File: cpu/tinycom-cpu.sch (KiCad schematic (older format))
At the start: 10 parts, among them P1 CONN_02X08, P2 CONN_02X08, U1 OLIMEX_IC_A13, U2 H5TQ2G83BFR/FBGA82, Y1 Crystal

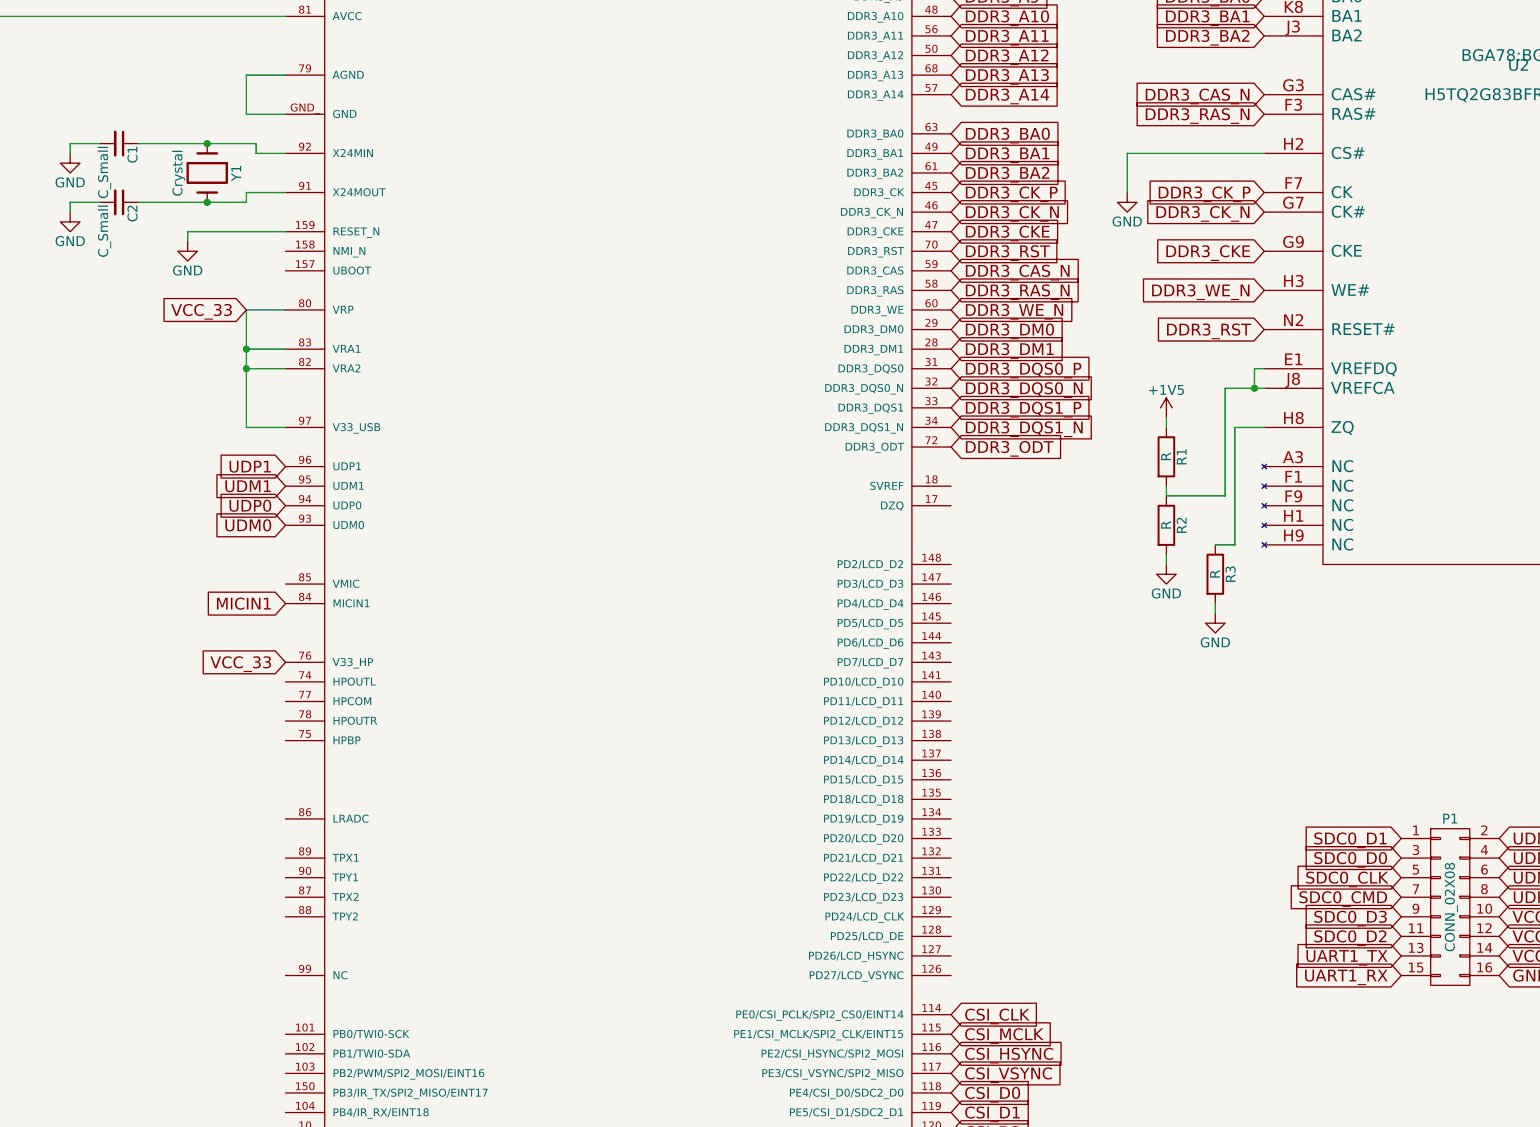
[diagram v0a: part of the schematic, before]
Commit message: router power
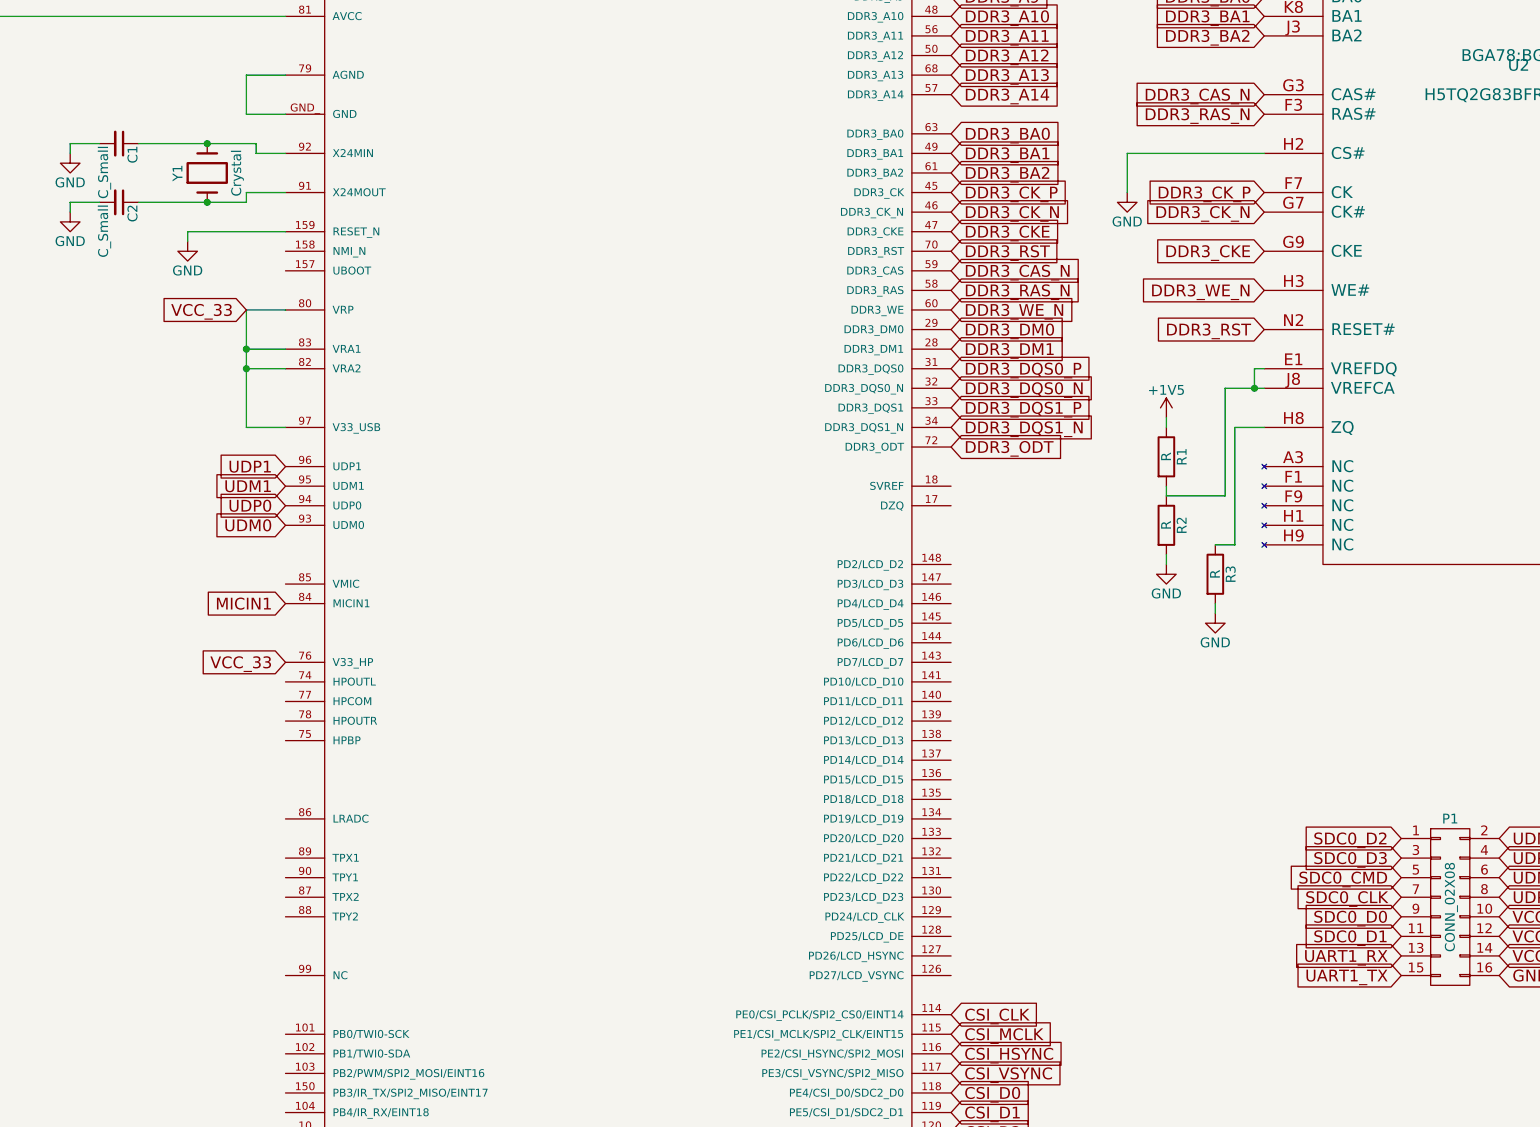
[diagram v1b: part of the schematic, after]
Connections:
- net SDC0_CLK: now also P1.7 (P7); no longer P1.5 (P5)
- net SDC0_CMD: now also P1.5 (P5); no longer P1.7 (P7)
- net SDC0_D0: now also P1.9 (P9); no longer P1.3 (P3)
- net SDC0_D1: now also P1.11 (P11); no longer P1.1 (P1)
- net SDC0_D2: now also P1.1 (P1); no longer P1.11 (P11)
- net SDC0_D3: now also P1.3 (P3); no longer P1.9 (P9)
- net UART1_RX: now also P1.13 (P13); no longer P1.15 (P15)
- net UART1_TX: now also P1.15 (P15); no longer P1.13 (P13)
- net at C2.1, U1.91 (X24MOUT): now also Y1.1; no longer Y1.2
- net at C1.1, U1.92 (X24MIN): now also Y1.2; no longer Y1.1
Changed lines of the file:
@@
 UDM0
 Text GLabel 7350 5400 0    60   Input ~ 0
+SDC0_D2
+Text GLabel 7350 5500 0    60   Input ~ 0
+SDC0_D3
+Text GLabel 7350 5600 0    60   Input ~ 0
+SDC0_CMD
+Text GLabel 7350 5700 0    60   Input ~ 0
+SDC0_CLK
+Text GLabel 7350 5800 0    60   Input ~ 0
+SDC0_D0
+Text GLabel 7350 5900 0    60   Input ~ 0
 SDC0_D1
-Text GLabel 7350 5500 0    60   Input ~ 0
-SDC0_D0
-Text GLabel 7350 5600 0    60   Input ~ 0
-SDC0_CLK
-Text GLabel 7350 5700 0    60   Input ~ 0
-SDC0_CMD
-Text GLabel 7350 5800 0    60   Input ~ 0
-SDC0_D3
-Text GLabel 7350 5900 0    60   Input ~ 0
-SDC0_D2
 Text GLabel 7850 5400 2    60   Input ~ 0
 UDM0
@@
 CSI_D7
 Text GLabel 7350 6000 0    60   Input ~ 0
+UART1_RX
+Text GLabel 7350 6100 0    60   Input ~ 0
 UART1_TX
-Text GLabel 7350 6100 0    60   Input ~ 0
-UART1_RX
 Text GLabel 9400 6100 2    60   Input ~ 0
 GND
@@
 F 3 "" H 1250 2000 60  0000 C CNN
 	1    1250 2000
-	0    1    1    0
+	0    -1   -1   0
 $EndComp
 $Comp
@@
 	1500 1900 1500 1850
 Wire Wire Line
-	1500 1850 900  1850
-Wire Wire Line
 	1650 2100 1450 2100
 Wire Wire Line
-	1450 2100 1450 2150
-Wire Wire Line
-	1450 2150 900  2150
+	1450 2150 1450 2100
 Connection ~ 1250 1850
 Connection ~ 1250 2150
@@
 Wire Wire Line
 	6400 4200 6400 4250
+Wire Wire Line
+	1500 1850 900  1850
+Wire Wire Line
+	900  2150 1450 2150
 $EndSCHEMATC
